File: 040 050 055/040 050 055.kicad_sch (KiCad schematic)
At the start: 7 parts, among them J05x1 05x, J40 040

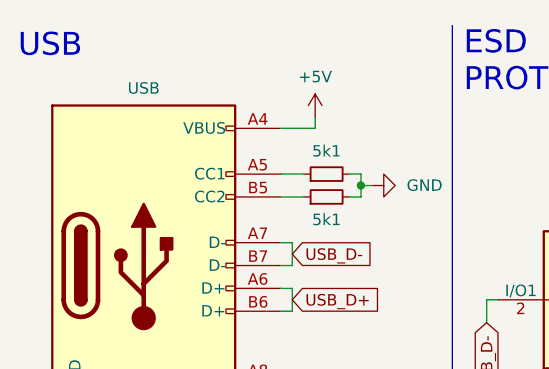
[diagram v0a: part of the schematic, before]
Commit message: Unknown Changes
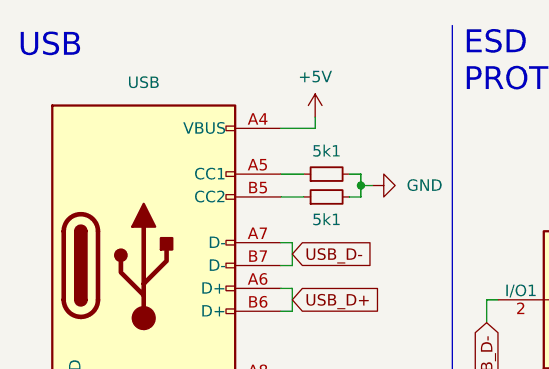
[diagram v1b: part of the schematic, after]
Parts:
- JUSB1: footprint (none) -> Connector_Custom:YTC-16S-28
- LED1: footprint (none) -> LED_Custom:FM-3510RGBA-SG
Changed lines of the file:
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@@
       (effects (font (size 1.27 1.27)))
     )
-    (property "Footprint" "" (at 118.11 41.91 0)
+    (property "Footprint" "LED_Custom:FM-3510RGBA-SG" (at 118.11 41.91 0)
       (effects (font (size 1.27 1.27)) hide)
     )
@@
       (effects (font (size 1.27 1.27)) hide)
     )
-    (property "Value" "USB" (at 26.67 19.685 0)
+    (property "Value" "USB" (at 26.67 19.05 0)
       (effects (font (size 1.27 1.27)))
     )
-    (property "Footprint" "" (at 30.48 39.37 0)
+    (property "Footprint" "Connector_Custom:YTC-16S-28" (at 30.48 39.37 0)
       (effects (font (size 1.27 1.27)) hide)
     )
